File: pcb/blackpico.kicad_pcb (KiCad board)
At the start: 2 copper layers, 53.3 x 31.8 mm, 3 parts, among them U1 RP2040

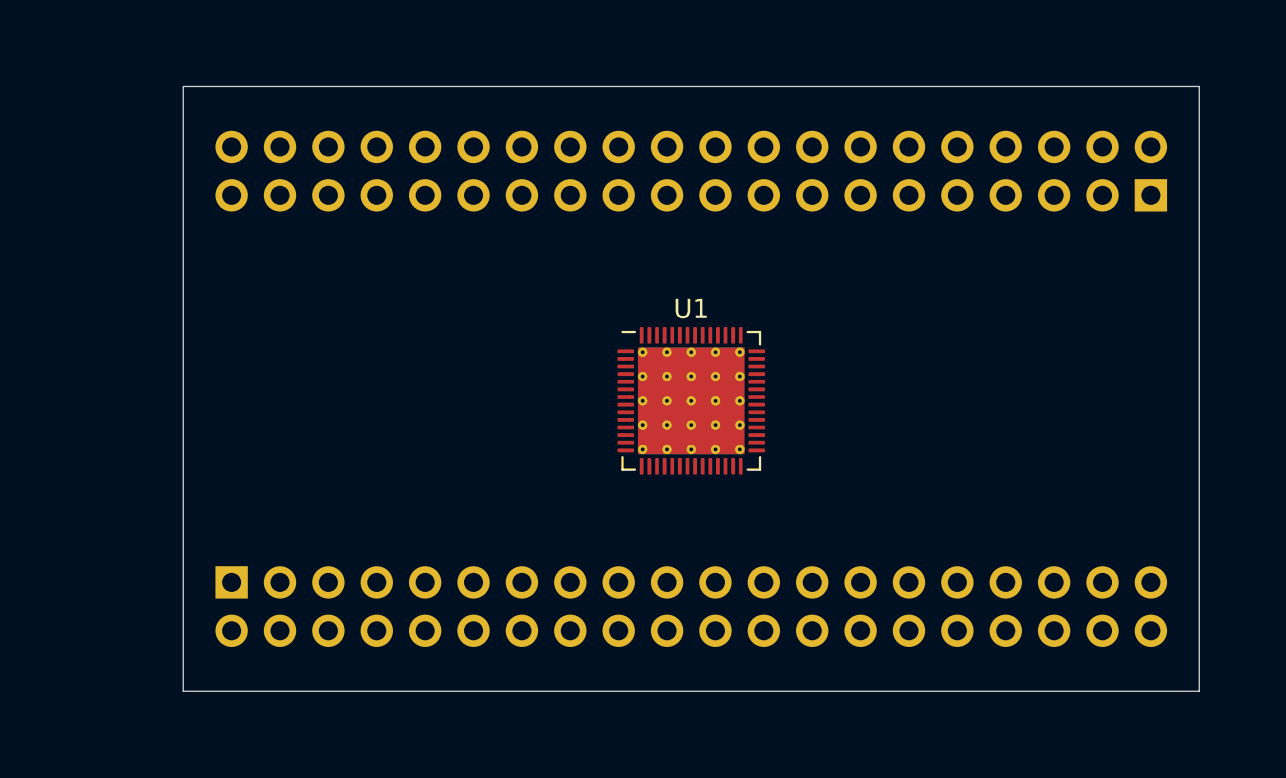
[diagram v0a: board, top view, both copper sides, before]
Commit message: Hmmmm
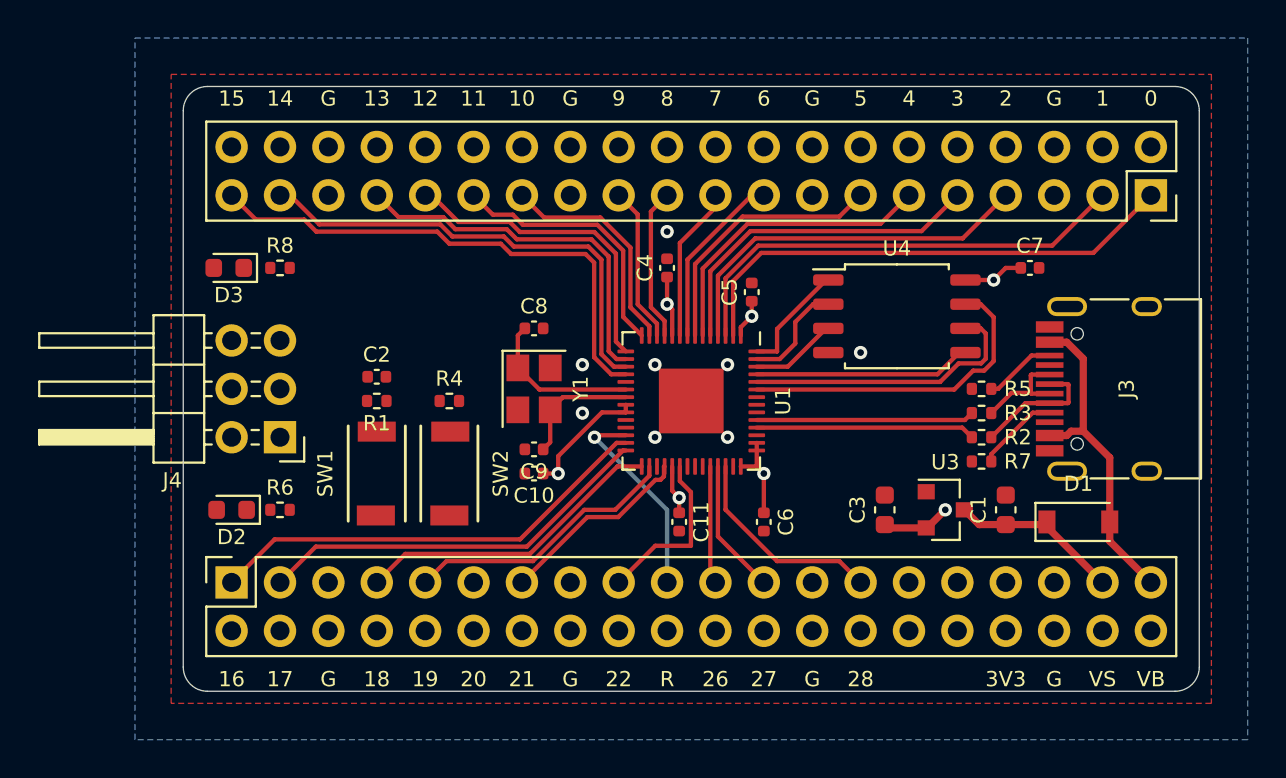
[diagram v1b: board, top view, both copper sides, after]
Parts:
- added C1: 10uF, Capacitor_SMD:C_0603_1608Metric, F.Cu at (200.7, 118.1)
- added C10: 100nF, Capacitor_SMD:C_0402_1005Metric, F.Cu at (175.9, 116.2)
- added C11: 100nF, Capacitor_SMD:C_0402_1005Metric, F.Cu at (183.5, 118.7)
- added C2: 100nF, Capacitor_SMD:C_0402_1005Metric, F.Cu at (167.6, 111.1)
- added C3: 10uF, Capacitor_SMD:C_0603_1608Metric, F.Cu at (194.3, 118.1)
- added C4: 100nF, Capacitor_SMD:C_0402_1005Metric, F.Cu at (182.9, 105.4)
- added C5: 100nF, Capacitor_SMD:C_0402_1005Metric, F.Cu at (187.3, 106.7)
- added C6: 100nF, Capacitor_SMD:C_0402_1005Metric, F.Cu at (188.0, 118.7)
- added C7: 100nF, Capacitor_SMD:C_0402_1005Metric, F.Cu at (201.9, 105.4)
- added C8: 15pF, Capacitor_SMD:C_0402_1005Metric, F.Cu at (175.9, 108.6)
- added C9: 15pF, Capacitor_SMD:C_0402_1005Metric, F.Cu at (175.9, 114.9)
- added D1: ~, Diode_SMD:D_SOD-123, F.Cu at (204.5, 118.7)
- added D2: GRE, LED_SMD:LED_0603_1608Metric, F.Cu at (160.0, 118.1)
- added D3: BLUE, LED_SMD:LED_0603_1608Metric, F.Cu at (159.9, 105.4)
- added J3: USB-C, blackpico:USB_C_Receptacle_HRO_TYPE-C-31-M-12, F.Cu at (207.0, 111.8)
- added J4: ~, Connector_PinHeader_2.54mm:PinHeader_2x03_P2.54mm_Horizontal, F.Cu at (162.6, 114.3)
- added R1: 10k, Resistor_SMD:R_0402_1005Metric, F.Cu at (167.6, 112.4)
- added R2: 22R, Resistor_SMD:R_0402_1005Metric, F.Cu at (199.4, 114.3)
- added R3: 22R, Resistor_SMD:R_0402_1005Metric, F.Cu at (199.4, 113.0)
- added R4: 10k, Resistor_SMD:R_0402_1005Metric, F.Cu at (171.4, 112.4)
- added R5: 5.1k, Resistor_SMD:R_0402_1005Metric, F.Cu at (199.4, 111.8)
- added R6: 220, Resistor_SMD:R_0402_1005Metric, F.Cu at (162.6, 118.1)
- added R7: 5.1k, Resistor_SMD:R_0402_1005Metric, F.Cu at (199.4, 115.6)
- added R8: 220, Resistor_SMD:R_0402_1005Metric, F.Cu at (162.6, 105.4)
- added SW1: TS-1088R-02526, blackpico:TS-1088R-02526, F.Cu at (167.6, 116.2)
- added SW2: TS-1088R-02526, blackpico:TS-1088R-02526, F.Cu at (171.4, 116.2)
- added U3: XC6206P332MR, Package_TO_SOT_SMD:SOT-23, F.Cu at (197.5, 118.1)
- added U4: W25Q32JVSS, Package_SO:SOIC-8_5.23x5.23mm_P1.27mm, F.Cu at (194.9, 108.0)
- added Y1: 12MHz, Crystal:Crystal_SMD_3225-4Pin_3.2x2.5mm, F.Cu at (175.9, 111.8)
- J1, J2: footprint Connector_PinHeader_2.54mm:PinHeader_2x20_P2.54mm_Vertical -> blackpico:PinSocket_2x20_P2.54mm_Vertical_Stackable; moved to F.Cu
- U1: footprint Package_DFN_QFN:QFN-56-1EP_7x7mm_P0.4mm_EP5.6x5.6mm_ThermalVias -> blackpico:QFN-56-1EP_7x7mm_P0.4mm_EP3.4x3.4mm
- moved J1 52.4 mm to (208.3, 101.6)
- moved J2 52.4 mm to (160.0, 121.9)
- turned U1 to 270 degrees
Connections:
- J1 pad 1: Net-(J1-Pad1) -> IO0
- J1 pad 10: Net-(J1-Pad10) -> IO3
- J1 pad 11: Net-(J1-Pad11) -> IO4
- J1 pad 12: Net-(J1-Pad12) -> IO4
- J1 pad 13: Net-(J1-Pad13) -> IO5
- J1 pad 14: Net-(J1-Pad14) -> IO5
- J1 pad 15: Net-(J1-Pad15) -> GND
- J1 pad 16: Net-(J1-Pad16) -> GND
- J1 pad 17: Net-(J1-Pad17) -> IO6
- J1 pad 18: Net-(J1-Pad18) -> IO6
- J1 pad 19: Net-(J1-Pad19) -> IO7
- J1 pad 2: Net-(J1-Pad2) -> IO0
- J1 pad 20: Net-(J1-Pad20) -> IO7
- J1 pad 21: Net-(J1-Pad21) -> IO8
- J1 pad 22: Net-(J1-Pad22) -> IO8
- J1 pad 23: Net-(J1-Pad23) -> IO9
- J1 pad 24: Net-(J1-Pad24) -> IO9
- J1 pad 25: Net-(J1-Pad25) -> GND
- J1 pad 26: Net-(J1-Pad26) -> GND
- J1 pad 27: Net-(J1-Pad27) -> IO10
- J1 pad 28: Net-(J1-Pad28) -> IO10
- J1 pad 29: Net-(J1-Pad29) -> IO11
- J1 pad 3: Net-(J1-Pad3) -> IO1
- J1 pad 30: Net-(J1-Pad30) -> IO11
- J1 pad 31: Net-(J1-Pad31) -> IO12
- J1 pad 32: Net-(J1-Pad32) -> IO12
- J1 pad 33: Net-(J1-Pad33) -> IO13
- J1 pad 34: Net-(J1-Pad34) -> IO13
- J1 pad 35: Net-(J1-Pad35) -> GND
- J1 pad 36: Net-(J1-Pad36) -> GND
- J1 pad 37: Net-(J1-Pad37) -> IO14
- J1 pad 38: Net-(J1-Pad38) -> IO14
- J1 pad 39: Net-(J1-Pad39) -> IO15
- J1 pad 4: Net-(J1-Pad4) -> IO1
- J1 pad 40: Net-(J1-Pad40) -> IO15
- J1 pad 5: Net-(J1-Pad5) -> GND
- J1 pad 6: Net-(J1-Pad6) -> GND
- J1 pad 7: Net-(J1-Pad7) -> IO2
- J1 pad 8: Net-(J1-Pad8) -> IO2
- J1 pad 9: Net-(J1-Pad9) -> IO3
- J2 pad 1: Net-(J2-Pad1) -> IO16
- J2 pad 10: Net-(J2-Pad10) -> IO19
- J2 pad 11: Net-(J2-Pad11) -> IO20
- J2 pad 12: Net-(J2-Pad12) -> IO20
- J2 pad 13: Net-(J2-Pad13) -> IO21
- J2 pad 14: Net-(J2-Pad14) -> IO21
- J2 pad 15: Net-(J2-Pad15) -> GND
- J2 pad 16: Net-(J2-Pad16) -> GND
- J2 pad 17: Net-(J2-Pad17) -> IO22
- J2 pad 18: Net-(J2-Pad18) -> IO22
- J2 pad 19: Net-(J2-Pad19) -> RUN
- J2 pad 2: Net-(J2-Pad2) -> IO16
- J2 pad 20: Net-(J2-Pad20) -> RUN
- J2 pad 21: Net-(J2-Pad21) -> IO26
- J2 pad 22: Net-(J2-Pad22) -> IO26
- J2 pad 23: Net-(J2-Pad23) -> IO27
- J2 pad 24: Net-(J2-Pad24) -> IO27
- J2 pad 25: Net-(J2-Pad25) -> GND
- J2 pad 26: Net-(J2-Pad26) -> GND
- J2 pad 27: Net-(J2-Pad27) -> IO28
- J2 pad 28: Net-(J2-Pad28) -> IO28
- J2 pad 3: Net-(J2-Pad3) -> IO17
- J2 pad 30: Net-(J2-Pad30) -> Net-(J2-Pad29)
- J2 pad 32: Net-(J2-Pad32) -> Net-(J2-Pad31)
- J2 pad 33: Net-(J2-Pad33) -> +3V3
- J2 pad 34: Net-(J2-Pad34) -> +3V3
- J2 pad 35: Net-(J2-Pad35) -> GND
- J2 pad 36: Net-(J2-Pad36) -> GND
- J2 pad 37: Net-(J2-Pad37) -> VDC
- J2 pad 38: Net-(J2-Pad38) -> VDC
- J2 pad 39: Net-(J2-Pad39) -> VBUS
- J2 pad 4: Net-(J2-Pad4) -> IO17
- J2 pad 40: Net-(J2-Pad40) -> VBUS
- J2 pad 5: Net-(J2-Pad5) -> GND
- J2 pad 6: Net-(J2-Pad6) -> GND
- J2 pad 7: Net-(J2-Pad7) -> IO18
- J2 pad 8: Net-(J2-Pad8) -> IO18
- J2 pad 9: Net-(J2-Pad9) -> IO19
- U1 pad 1: Net-(U1-Pad1) -> +3V3
- U1 pad 10: Net-(U1-Pad10) -> +3V3
- U1 pad 11: Net-(U1-Pad11) -> IO8
- U1 pad 12: Net-(U1-Pad12) -> IO9
- U1 pad 13: Net-(U1-Pad13) -> IO10
- U1 pad 14: Net-(U1-Pad14) -> IO11
- U1 pad 15: Net-(U1-Pad15) -> IO12
- U1 pad 16: Net-(U1-Pad16) -> IO13
- U1 pad 17: Net-(U1-Pad17) -> IO14
- U1 pad 18: Net-(U1-Pad18) -> IO15
- U1 pad 19: Net-(U1-Pad19) -> GND
- U1 pad 2: Net-(U1-Pad2) -> IO0
- U1 pad 20: Net-(U1-Pad20) -> XI
- U1 pad 21: Net-(U1-Pad21) -> XO
- U1 pad 22: Net-(U1-Pad22) -> +3V3
- U1 pad 23: Net-(U1-Pad23) -> +3V3
- U1 pad 26: Net-(U1-Pad26) -> RUN
- U1 pad 27: Net-(U1-Pad27) -> IO16
- U1 pad 28: Net-(U1-Pad28) -> IO17
- U1 pad 29: Net-(U1-Pad29) -> IO18
- U1 pad 3: Net-(U1-Pad3) -> IO1
- U1 pad 30: Net-(U1-Pad30) -> IO19
- U1 pad 31: Net-(U1-Pad31) -> IO20
- U1 pad 32: Net-(U1-Pad32) -> IO21
- U1 pad 33: Net-(U1-Pad33) -> +3V3
- U1 pad 34: Net-(U1-Pad34) -> IO22
- U1 pad 38: Net-(U1-Pad38) -> IO26
- U1 pad 39: Net-(U1-Pad39) -> IO27
- U1 pad 4: Net-(U1-Pad4) -> IO2
- U1 pad 40: Net-(U1-Pad40) -> IO28
- U1 pad 42: Net-(U1-Pad42) -> +3V3
- U1 pad 43: Net-(U1-Pad43) -> +3V3
- U1 pad 44: Net-(U1-Pad44) -> +3V3
- U1 pad 46: Net-(U1-Pad46) -> D-
- U1 pad 47: Net-(U1-Pad47) -> D+
- U1 pad 5: Net-(U1-Pad5) -> IO3
- U1 pad 51: Net-(U1-Pad51) -> QD3
- U1 pad 52: Net-(U1-Pad52) -> QCK
- U1 pad 53: Net-(U1-Pad53) -> QD0
- U1 pad 54: Net-(U1-Pad54) -> QD2
- U1 pad 55: Net-(U1-Pad55) -> QD1
- U1 pad 56: Net-(U1-Pad56) -> QSS
- U1 pad 57: Net-(U1-Pad57) -> GND
- U1 pad 6: Net-(U1-Pad6) -> IO4
- U1 pad 7: Net-(U1-Pad7) -> IO5
- U1 pad 8: Net-(U1-Pad8) -> IO6
- U1 pad 9: Net-(U1-Pad9) -> IO7
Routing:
- net IO15: track 0.00 -> 30.0 mm
- net +3V3: track 0.00 -> 29.2 mm, vias 0 -> 7
- net IO0: track 0.00 -> 29.2 mm
- net IO14: track 0.00 -> 27.3 mm
- net IO1: track 0.00 -> 27.1 mm
- net IO16: track 0.00 -> 26.3 mm
- net IO17: track 0.00 -> 23.6 mm
- net IO2: track 0.00 -> 22.5 mm
- net IO13: track 0.00 -> 22.1 mm
- net IO3: track 0.00 -> 20.5 mm
- net GND: track 0.00 -> 20.3 mm, vias 0 -> 8
- net VBUS: track 0.00 -> 19.7 mm
- net IO12: track 0.00 -> 19.2 mm
- net IO18: track 0.00 -> 19.0 mm
- net IO4: track 0.00 -> 18.5 mm
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- added copper zone on In1.Cu, net +3V3
- added copper zone on B.Cu, net GND
- added copper zone on F.Cu, net GND
- added copper zone on In2.Cu, net GND
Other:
- outline, holes or cut-outs redrawn
- copper layers 2 -> 4
- net class Default: clearance 0.2 -> 0.1524; trace_width 0.25 -> 0.1524; via_dia 0.8 -> 0.7; via_drill 0.4 -> 0.35
- rule trace_clearance: 0.2 -> 0.1524
- rule trace_min: 0.2 -> 0.1524
- board text added: "0"
- board text added: "1"
- board text added: "10"
- board text added: "11"
- board text added: "12"
- board text added: "13"
- board text added: "14"
- board text added: "15"
- board text added: "16"
- board text added: "17"
- board text added: "18"
- board text added: "19"
- board text added: "2"
- board text added: "20"
- board text added: "21"
- board text added: "22"
- board text added: "26"
- board text added: "27"
- board text added: "28"
- board text added: "3"
- board text added: "3V3"
- board text added: "4"
- board text added: "5"
- board text added: "6"
- board text added: "7"
- board text added: "8"
- board text added: "9"
- board text added: "G"
- board text added: "R"
- board text added: "VB"
- board text added: "VS"
